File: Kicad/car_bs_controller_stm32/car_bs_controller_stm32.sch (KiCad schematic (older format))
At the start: 2 parts

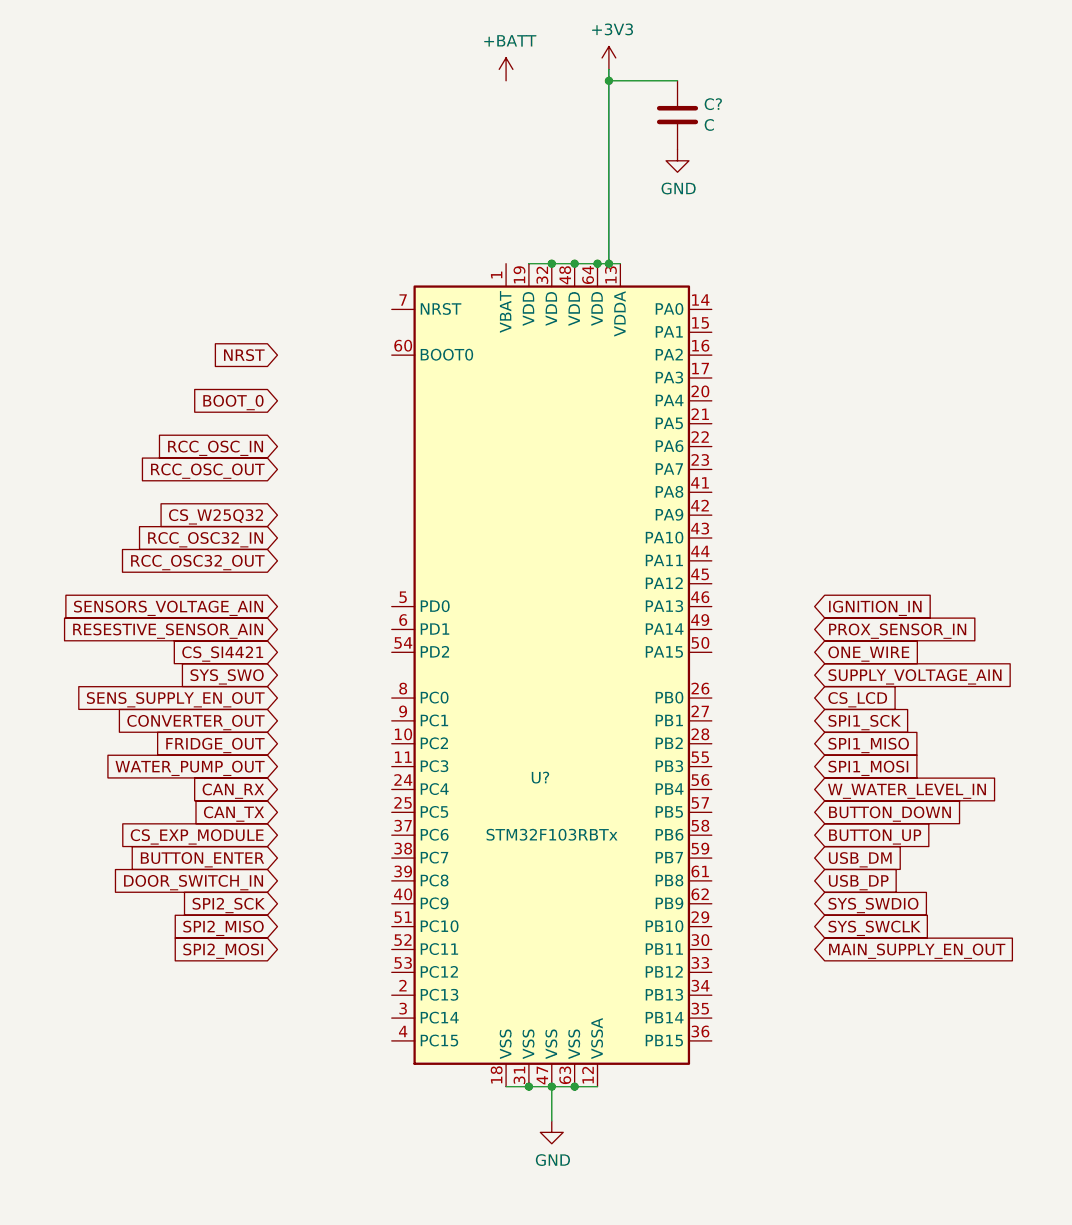
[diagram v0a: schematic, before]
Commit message: continued development
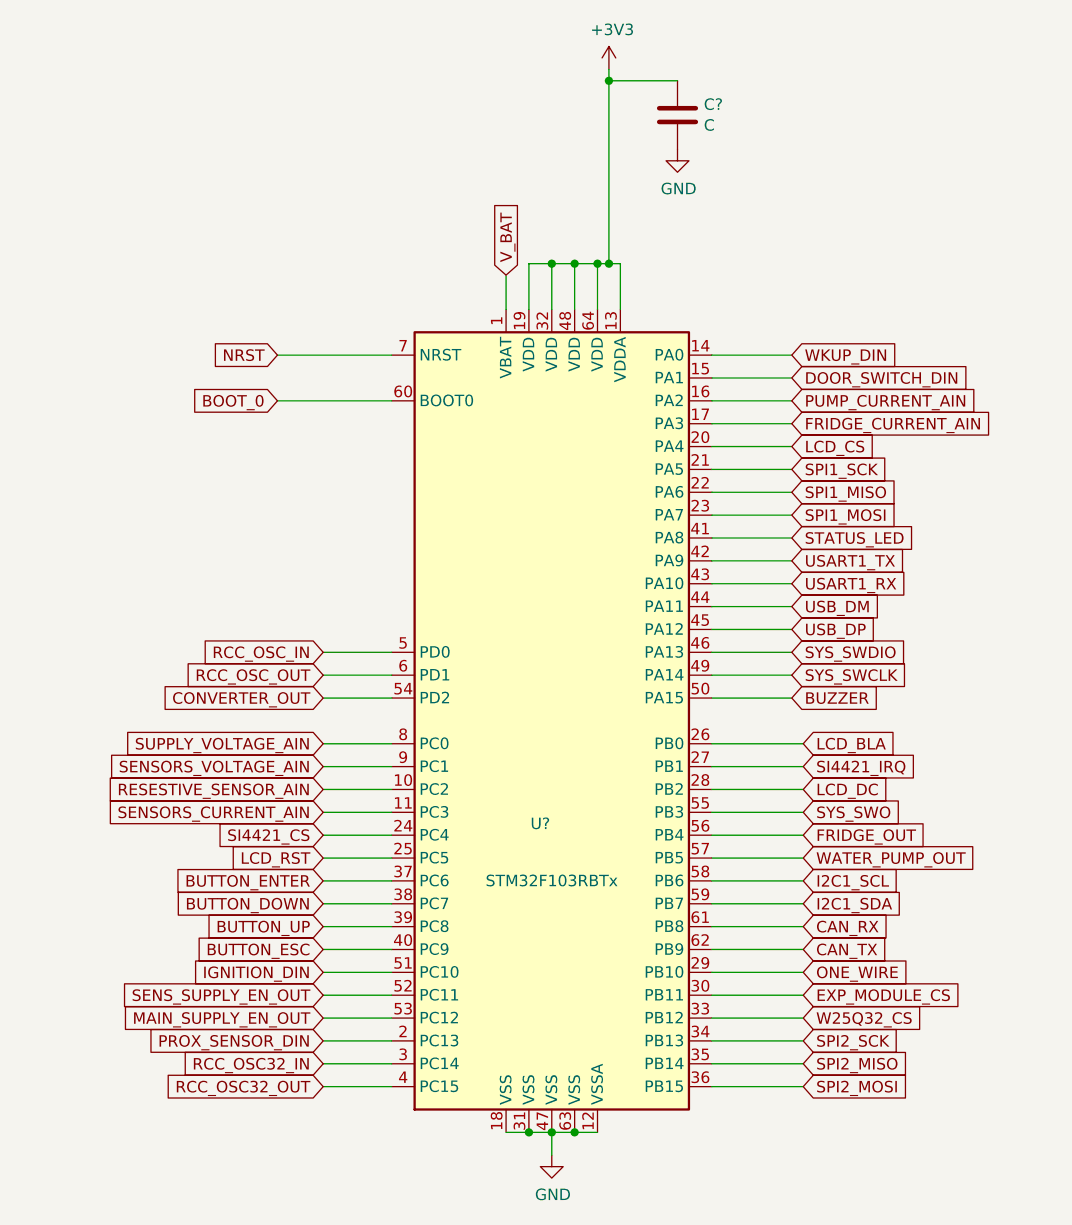
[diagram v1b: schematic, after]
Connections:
- net BOOT_0: now also U?.60 (BOOT0)
- net BUTTON_DOWN: now also U?.38 (PC7)
- net BUTTON_ENTER: now also U?.37 (PC6)
- net BUTTON_UP: now also U?.39 (PC8)
- net CAN_RX: now also U?.61 (PB8)
- net CAN_TX: now also U?.62 (PB9)
- net CONVERTER_OUT: now also U?.54 (PD2)
- net FRIDGE_OUT: now also U?.56 (PB4)
- net MAIN_SUPPLY_EN_OUT: now also U?.53 (PC12)
- net NRST: now also U?.7 (NRST)
- net ONE_WIRE: now also U?.29 (PB10)
- net RCC_OSC32_IN: now also U?.3 (PC14)
- net RCC_OSC32_OUT: now also U?.4 (PC15)
- net RCC_OSC_IN: now also U?.5 (PD0)
- net RCC_OSC_OUT: now also U?.6 (PD1)
- net RESESTIVE_SENSOR_AIN: now also U?.10 (PC2)
- net SENSORS_VOLTAGE_AIN: now also U?.9 (PC1)
- net SENS_SUPPLY_EN_OUT: now also U?.52 (PC11)
- net SPI1_MISO: now also U?.22 (PA6)
- net SPI1_MOSI: now also U?.23 (PA7)
- net SPI1_SCK: now also U?.21 (PA5)
- net SPI2_MISO: now also U?.35 (PB14)
- net SPI2_MOSI: now also U?.36 (PB15)
- net SPI2_SCK: now also U?.34 (PB13)
- net SUPPLY_VOLTAGE_AIN: now also U?.8 (PC0)
- net SYS_SWCLK: now also U?.49 (PA14)
- net SYS_SWDIO: now also U?.46 (PA13)
- net SYS_SWO: now also U?.55 (PB3)
- net USB_DM: now also U?.44 (PA11)
- net USB_DP: now also U?.45 (PA12)
- net WATER_PUMP_OUT: now also U?.57 (PB5)
- net V_BAT: now reaches U?.1 (VBAT)
- net SENSORS_CURRENT_AIN: now reaches U?.11 (PC3)
- net WKUP_DIN: now reaches U?.14 (PA0)
- net DOOR_SWITCH_DIN: now reaches U?.15 (PA1)
- net PUMP_CURRENT_AIN: now reaches U?.16 (PA2)
- net FRIDGE_CURRENT_AIN: now reaches U?.17 (PA3)
- net PROX_SENSOR_DIN: now reaches U?.2 (PC13)
- net LCD_CS: now reaches U?.20 (PA4)
- net SI4421_CS: now reaches U?.24 (PC4)
- net LCD_RST: now reaches U?.25 (PC5)
- net LCD_BLA: now reaches U?.26 (PB0)
- net SI4421_IRQ: now reaches U?.27 (PB1)
- net LCD_DC: now reaches U?.28 (PB2)
- net EXP_MODULE_CS: now reaches U?.30 (PB11)
- net W25Q32_CS: now reaches U?.33 (PB12)
- net BUTTON_ESC: now reaches U?.40 (PC9)
- net STATUS_LED: now reaches U?.41 (PA8)
- net USART1_TX: now reaches U?.42 (PA9)
- net USART1_RX: now reaches U?.43 (PA10)
- net BUZZER: now reaches U?.50 (PA15)
- net IGNITION_DIN: now reaches U?.51 (PC10)
- net I2C1_SCL: now reaches U?.58 (PB6)
- net I2C1_SDA: now reaches U?.59 (PB7)
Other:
- moved on the sheet: U?
